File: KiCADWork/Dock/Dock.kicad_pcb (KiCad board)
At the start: 2 copper layers, 166.3 x 101.1 mm, 11 parts, among them J1 Conn_01x10_Pin, J2 Conn_01x10_Pin, U1 MCP73831T-2ACI/OT, U2 XB6096I2SV

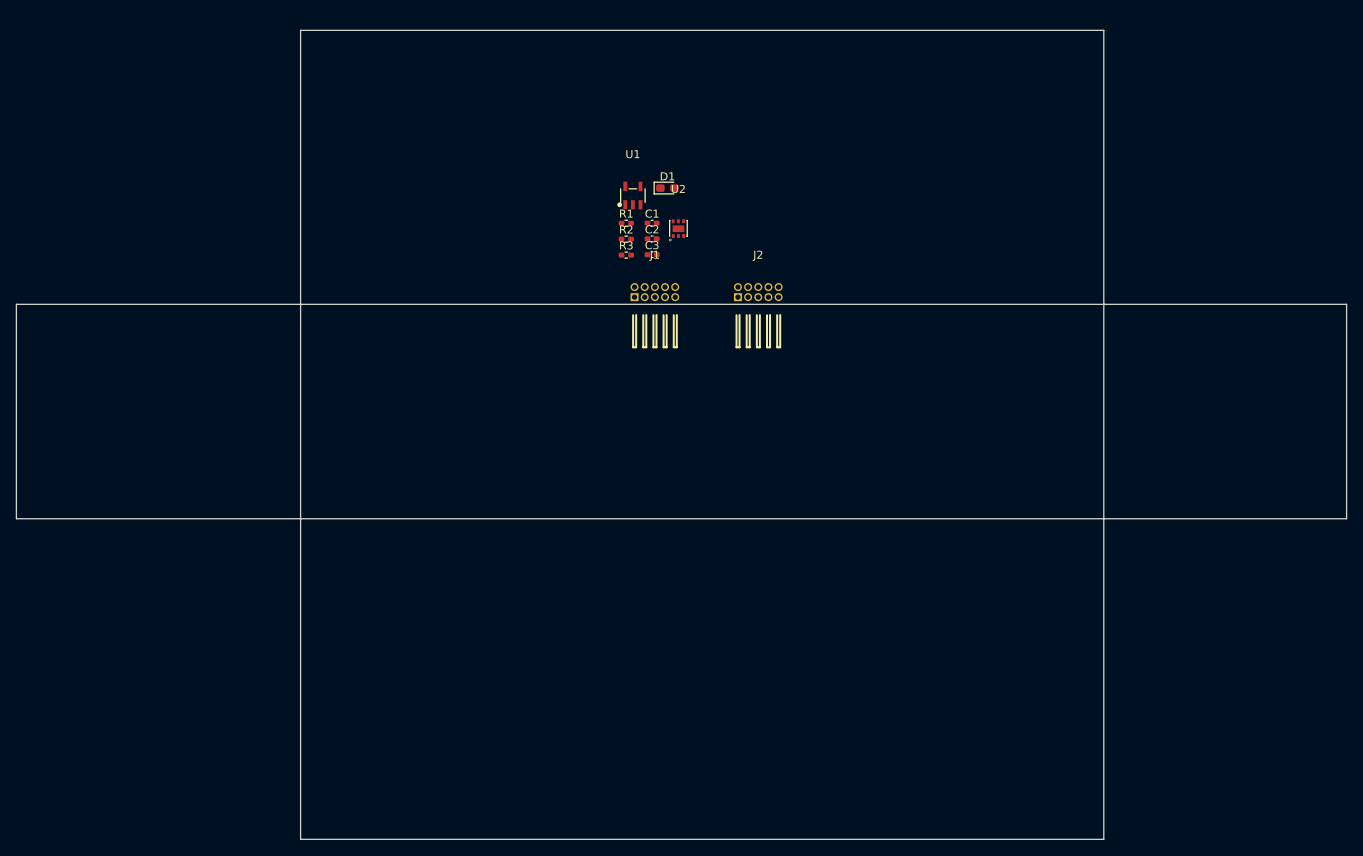
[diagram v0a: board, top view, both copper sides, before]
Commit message: Dock Updates
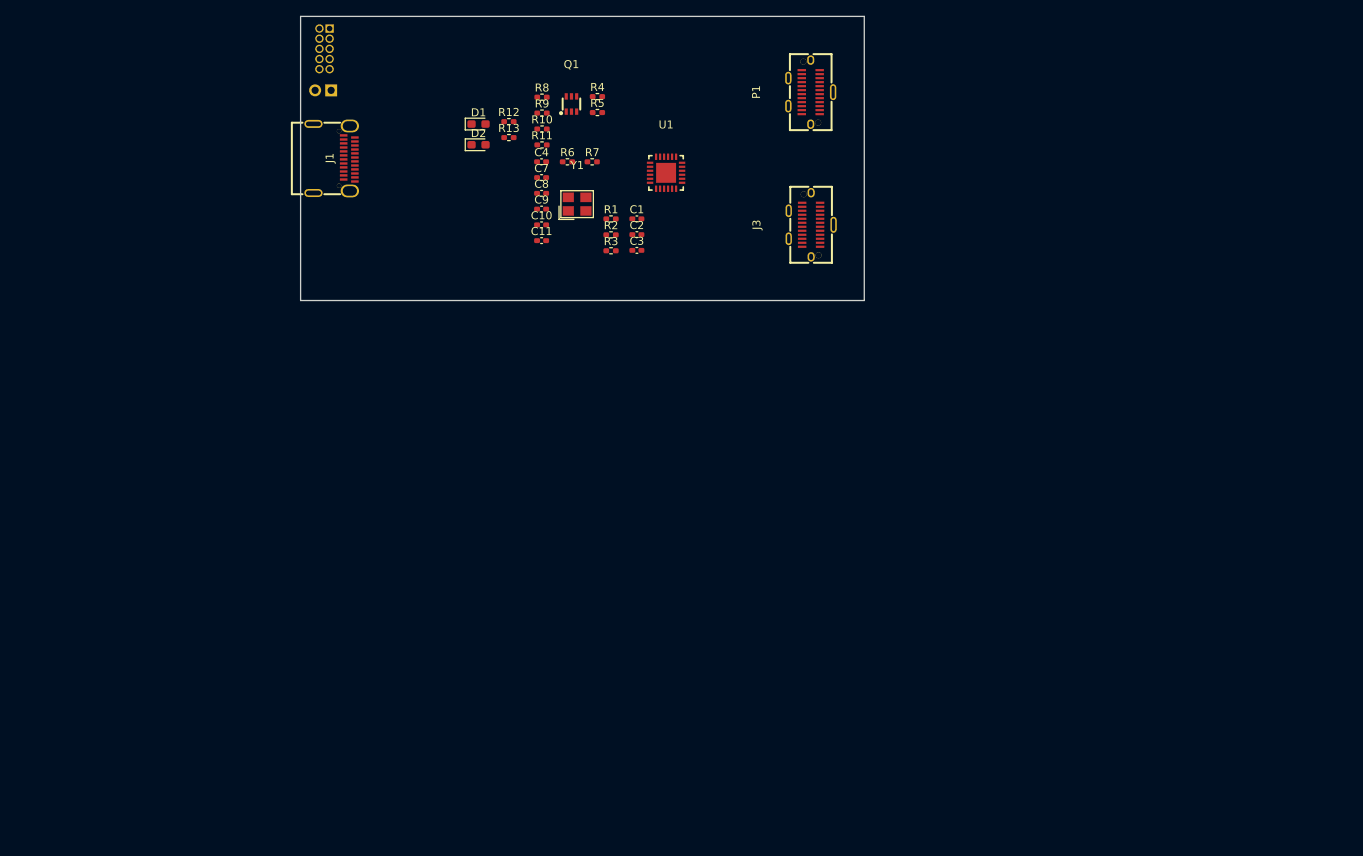
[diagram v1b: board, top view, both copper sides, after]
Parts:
- removed J2: Conn_01x10_Pin, easyeda2kicad:HDR-TH_10P-P1.27-H-M-R2-C7-S1.27-W7.5-N
- removed U2: XB6096I2SV, easyeda2kicad:WDFN-6_L2.0-W2.0-P0.65-BL-EP
- added BT1: Battery, easyeda2kicad:CONN-TH_S2B-PH-K-LF-SN, B.Cu at (124.1, 52.7)
- added C10: 100n, Capacitor_SMD:C_0402_1005Metric_Pad0.74x0.62mm_HandSolder, F.Cu at (152.9, 61.1)
- added C11: 1u, Capacitor_SMD:C_0402_1005Metric_Pad0.74x0.62mm_HandSolder, F.Cu at (152.9, 63.1)
- added C4: 1u, Capacitor_SMD:C_0402_1005Metric_Pad0.74x0.62mm_HandSolder, F.Cu at (152.9, 53.2)
- added C7: 100n, Capacitor_SMD:C_0402_1005Metric_Pad0.74x0.62mm_HandSolder, F.Cu at (152.9, 55.2)
- added C8: 1u, Capacitor_SMD:C_0402_1005Metric_Pad0.74x0.62mm_HandSolder, F.Cu at (152.9, 57.1)
- added C9: 100n, Capacitor_SMD:C_0402_1005Metric_Pad0.74x0.62mm_HandSolder, F.Cu at (152.9, 59.1)
- added D2: LED, LED_SMD:LED_0603_1608Metric_Pad1.05x0.95mm_HandSolder, F.Cu at (145.1, 51.1)
- added J3: USB_C_Receptacle, easyeda2kicad:USB-C-SMD_TYPEC-952-ACP24, F.Cu at (186.6, 61.1)
- added J4: Conn_01x10_Socket, easyeda2kicad:HDR-TH_10P-P1.27-V-M-R2-C5-S1.27-1, B.Cu at (125.8, 39.1)
- added P1: USB_C_Plug, easyeda2kicad:USB-C-SMD_TYPEC-952-ACP24, F.Cu at (186.6, 44.5)
- added Q1: NTJD4152PT1G, easyeda2kicad:SC-88-6_L2.0-W1.3-P0.65-LS2.1-BL, F.Cu at (156.7, 46.0)
- added R10: 2k, Resistor_SMD:R_0402_1005Metric_Pad0.72x0.64mm_HandSolder, F.Cu at (153.0, 49.1)
- added R11: 2k, Resistor_SMD:R_0402_1005Metric_Pad0.72x0.64mm_HandSolder, F.Cu at (153.0, 51.1)
- added R12: 220, Resistor_SMD:R_0402_1005Metric_Pad0.72x0.64mm_HandSolder, F.Cu at (148.9, 48.2)
- added R13: 220, Resistor_SMD:R_0402_1005Metric_Pad0.72x0.64mm_HandSolder, F.Cu at (148.9, 50.2)
- added R4: 5k1, Resistor_SMD:R_0402_1005Metric_Pad0.72x0.64mm_HandSolder, F.Cu at (159.9, 45.1)
- added R5: 5k1, Resistor_SMD:R_0402_1005Metric_Pad0.72x0.64mm_HandSolder, F.Cu at (159.9, 47.0)
- added R6: 100, Resistor_SMD:R_0402_1005Metric_Pad0.72x0.64mm_HandSolder, F.Cu at (156.2, 53.2)
- added R7: 100, Resistor_SMD:R_0402_1005Metric_Pad0.72x0.64mm_HandSolder, F.Cu at (159.3, 53.2)
- added R8: 100, Resistor_SMD:R_0402_1005Metric_Pad0.72x0.64mm_HandSolder, F.Cu at (153.0, 45.1)
- added R9: 12k 1%, Resistor_SMD:R_0402_1005Metric_Pad0.72x0.64mm_HandSolder, F.Cu at (153.0, 47.1)
- added Y1: X322524MOB4SI, easyeda2kicad:CRYSTAL-SMD_4P-L3.2-W2.5-BL, F.Cu at (157.4, 58.5)
- C1: value 10u -> 18p
- C2: value 100n -> 18p
- C3: value 10u -> 100n
- D1: value WHITE LED -> LED
- J1: value Conn_01x10_Pin -> USB_C_Receptacle; footprint easyeda2kicad:HDR-TH_10P-P1.27-H-M-R2-C7-S1.27-W7.5-N -> easyeda2kicad:TYPE-C-SMD_C9900025773
- R1: value 2k -> 100
- R3: value 2k -> 10k
- U1: value MCP73831T-2ACI/OT -> USB2422T-I/MJ; footprint easyeda2kicad:SOT-23-5_L3.0-W1.7-P0.95-LS2.8-BL -> Temp:QFN-24_L4.0-W4.0-P0.50-TL-EP2.5
- moved J1 43.4 mm to (127.0, 52.8), turned to -90 degrees
- moved D1 24.9 mm to (145.1, 48.5)
- moved U1 5.04 mm to (168.5, 54.6)
- moved R3 1.98 mm to (161.6, 64.3)
- moved R1 1.98 mm to (161.6, 60.4)
- moved R2 1.98 mm to (161.6, 62.3)
- moved C1 1.98 mm to (164.9, 60.3)
- moved C2 1.98 mm to (164.9, 62.3)
- moved C3 1.98 mm to (164.9, 64.3)
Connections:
- C1 pad 1: +BATT -> GND
- C1 pad 2: GND -> Net-(U1-XTALIN/CLKIN)
- C2 pad 1: Net-(U2-VDD) -> Net-(U1-XTALOUT/(CLKIN_EN))
- C2 pad 2: /Charging/BATGND -> GND
- C3 pad 1: /Charging/VBUS -> GND
- C3 pad 2: GND -> +3V3
- D1 pad 1: Net-(D1-K) -> GND
- D1 pad 2: /Charging/VBUS -> Net-(D1-A)
- J1 pad 1: unconnected-(J1-Pin_1-Pad1) -> (no net)
- J1 pad 2: unconnected-(J1-Pin_2-Pad2) -> (no net)
- J1 pad 3: unconnected-(J1-Pin_3-Pad3) -> (no net)
- J1 pad 4: unconnected-(J1-Pin_4-Pad4) -> (no net)
- R1 pad 1: Net-(D1-K) -> Net-(U1-VBUS_DET)
- R1 pad 2: Net-(U1-STAT) -> VTRef
- R2 pad 1: Net-(U2-VDD) -> GND
- R2 pad 2: +BATT -> Net-(U1-VBUS_DET)
- R3 pad 1: Net-(U1-PROG) -> RESET
- R3 pad 2: GND -> +3V3
- U1 pad 1: Net-(U1-STAT) -> +3V3
- U1 pad 2: GND -> /DeviceSelect/D1-
- U1 pad 3: +BATT -> /DeviceSelect/D1+
- U1 pad 4: /Charging/VBUS -> /DeviceSelect/D2-
- U1 pad 5: Net-(U1-PROG) -> /DeviceSelect/D2+
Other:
- board size 166.3 x 101.1 mm -> 70.5 x 35.5 mm
